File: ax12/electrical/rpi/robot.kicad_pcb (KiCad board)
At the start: 2 copper layers, 99.1 x 47 mm, 38 parts, among them J1 12V, J2 LEG1, J3 Pi USB Pwr, J4 Serial, J5 LEG2, J6 LEG3, J7 LEG4, J8 Data P, J9 Data S, U1 LM317_12, U2 AP1117-50, U3 74LS126, U4 LM317_34

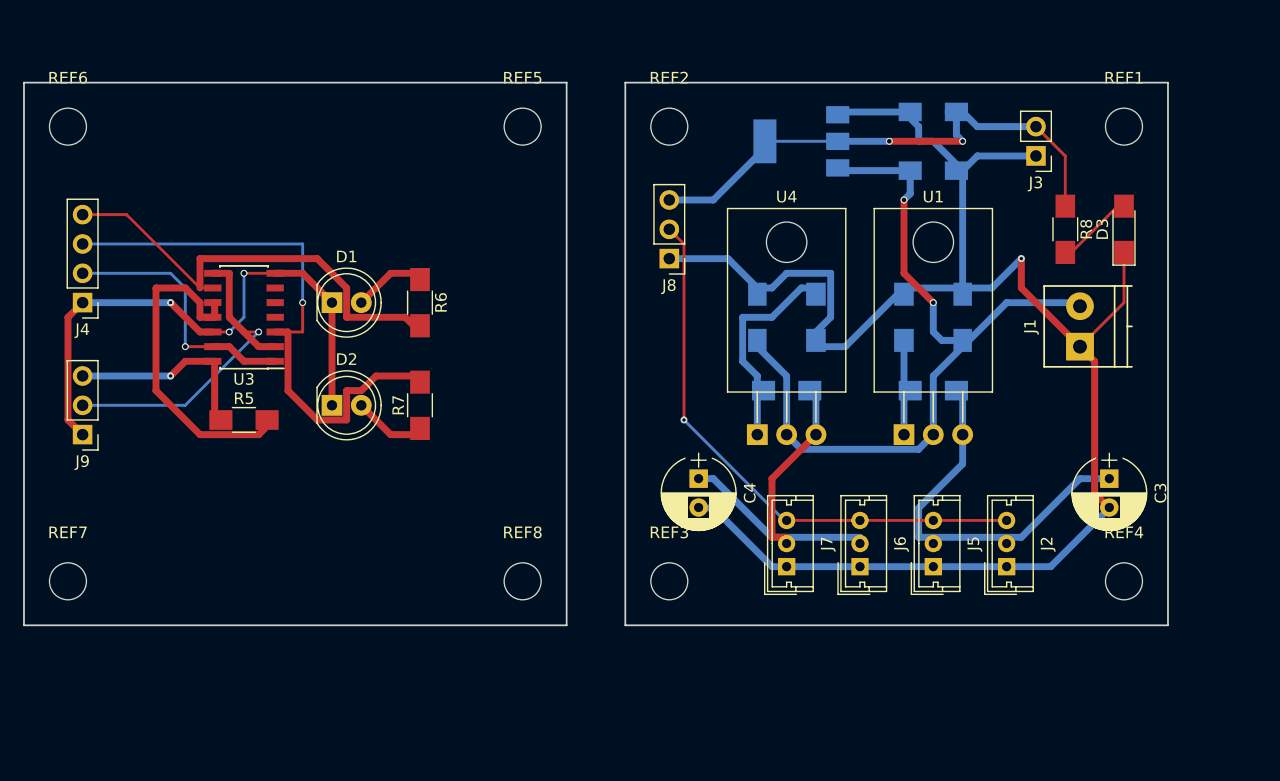
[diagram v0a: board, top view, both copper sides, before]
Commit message: update
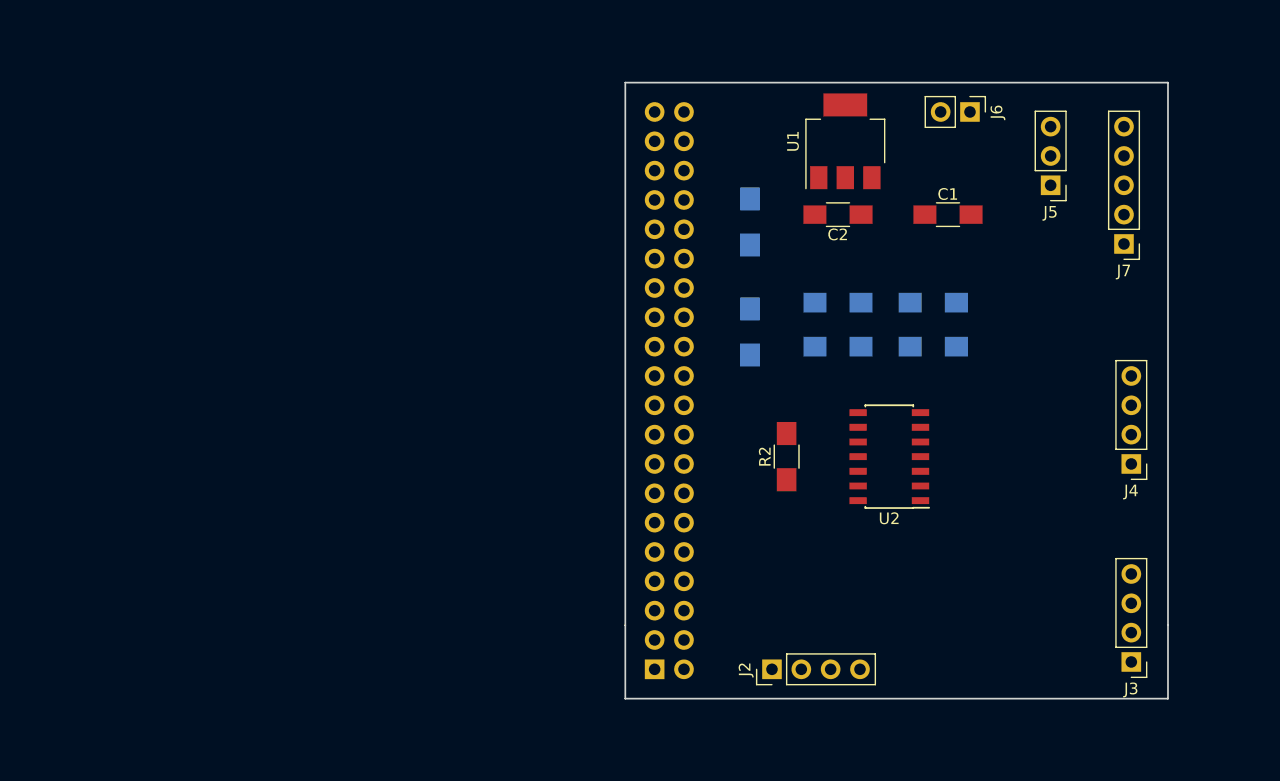
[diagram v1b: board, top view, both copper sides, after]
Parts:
- removed C3, C4: .1, Capacitors_THT:CP_Radial_D6.3mm_P2.50mm
- removed C5, C6: C, Capacitors_SMD:C_1206_HandSoldering
- removed J8: Data P, Pin_Headers:Pin_Header_Straight_1x03_Pitch2.54mm
- removed J9: Data S, Pin_Headers:Pin_Header_Straight_1x03_Pitch2.54mm
- removed R5: 10k, Resistors_SMD:R_1206_HandSoldering
- removed R6, R7, R8: 330, Resistors_SMD:R_1206_HandSoldering
- removed REF1, REF2, REF3, REF5, REF6, REF7, REF8: , Mounting_Holes:MountingHole_3.2mm_M3
- removed REF4: 3.2mm_M3, Mounting_Holes:MountingHole_3.2mm_M3
- removed U3: 74LS126, Housings_SOIC:SOIC-14_3.9x8.7mm_Pitch1.27mm
- removed U4: LM317_34, TO_SOT_Packages_THT:TO-220-3_Horizontal
- C1, C2: moved to F.Cu
- D1: value TX -> PWR; footprint LEDs:LED_D5.0mm -> LEDs:LED_1206_HandSoldering; moved to B.Cu
- D2: value RX -> TX; footprint LEDs:LED_D5.0mm -> LEDs:LED_1206_HandSoldering; moved to B.Cu
- D3: value PWR -> RX; moved to B.Cu
- J1: value 12V -> (none); footprint TerminalBlocks_Phoenix:TerminalBlock_Phoenix_PT-3.5mm_2pol -> Pin_Headers:Pin_Header_Straight_2x20_Pitch2.54mm; moved to B.Cu
- J2: value LEG1 -> IMU; footprint Connectors_Molex:Molex_MicroLatch-53253-0370_03x2.00mm_Straight -> Pin_Headers:Pin_Header_Straight_1x04_Pitch2.54mm
- J3: value Pi USB Pwr -> Lidar; footprint Pin_Headers:Pin_Header_Straight_1x02_Pitch2.54mm -> Pin_Headers:Pin_Header_Straight_1x04_Pitch2.54mm
- J5: value LEG2 -> Data S; footprint Connectors_Molex:Molex_MicroLatch-53253-0370_03x2.00mm_Straight -> Pin_Headers:Pin_Header_Straight_1x03_Pitch2.54mm
- J6: value LEG3 -> Pi USB Pwr; footprint Connectors_Molex:Molex_MicroLatch-53253-0370_03x2.00mm_Straight -> Pin_Headers:Pin_Header_Straight_1x02_Pitch2.54mm
- J7: value LEG4 -> Audio; footprint Connectors_Molex:Molex_MicroLatch-53253-0370_03x2.00mm_Straight -> Pin_Headers:Pin_Header_Straight_1x05_Pitch2.54mm
- R2: value 1.8k -> 10k; moved to F.Cu
- R4: value 1.8k -> 330
- U1: value LM317_12 -> AP1117-50; footprint TO_SOT_Packages_THT:TO-220-3_Horizontal -> TO_SOT_Packages_SMD:SOT-223-3_TabPin2
- U2: value AP1117-50 -> 74LS126; footprint TO_SOT_Packages_SMD:SOT-223-3_TabPin2 -> Housings_SOIC:SOIC-14_3.9x8.7mm_Pitch1.27mm; moved to F.Cu
- moved J4 91.9 mm to (153.0, 92.7)
- moved J1 46.2 mm to (111.8, 110.5), turned to 0 degrees
- moved D2 44.7 mm to (127.6, 78.7)
- moved J3 44.6 mm to (153.0, 109.9)
- moved J6 40.5 mm to (139.1, 62.2), turned to 270 degrees
- moved J7 40.4 mm to (152.4, 73.7), turned to 180 degrees
- moved D1 36.9 mm to (120.0, 71.8), turned to 270 degrees
- moved J5 34.5 mm to (146.1, 68.6), turned to 180 degrees
- moved U2 28.3 mm to (132.1, 92.1)
- moved D3 26.8 mm to (127.6, 82.5), turned to 0 degrees
- moved U1 25.9 mm to (128.3, 64.8), turned to 90 degrees
- moved J2 22.2 mm to (121.9, 110.5)
- moved R1 16.7 mm to (120.0, 81.3), turned to 90 degrees
- moved R2 15.8 mm to (123.2, 92.1)
- moved R3 14.8 mm to (135.9, 78.7), turned to 0 degrees
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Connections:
- C1 pad 2: GNDA -> GND
- C2 pad 2: GNDA -> GND
- D3 pad 1: GNDA -> GND
- J1 pad 1: GNDA -> Net-(J1-Pad1)
- J1 pad 2: +12V -> Net-(J1-Pad2)
- J2 pad 1: GNDA -> Net-(J1-Pad17)
- J2 pad 2: /PWR12 -> Net-(J1-Pad3)
- J2 pad 3: /DATA -> Net-(J1-Pad5)
- J3 pad 1: GNDA -> +5V
- J3 pad 2: +5V -> Net-(J1-Pad8)
- J5 pad 1: GNDA -> GND
- J5 pad 2: /PWR12 -> Net-(J5-Pad2)
- J5 pad 3: /DATA -> +12V
- J6 pad 1: GNDA -> GND
- J6 pad 2: /PWR34 -> +5V
- J7 pad 1: GNDA -> Net-(J7-Pad1)
- J7 pad 2: /PWR34 -> Net-(J7-Pad2)
- J7 pad 3: /DATA -> Net-(J7-Pad3)
- R1 pad 1: /PWR12 -> +5V
- R1 pad 2: Net-(R1-Pad2) -> Net-(D1-Pad2)
- R2 pad 1: Net-(R1-Pad2) -> +5V
- R2 pad 2: GNDA -> Net-(R2-Pad2)
- R3 pad 1: /PWR34 -> Net-(D2-Pad2)
- R3 pad 2: Net-(R3-Pad2) -> /TXI
- R4 pad 1: Net-(R3-Pad2) -> Net-(D3-Pad2)
- R4 pad 2: GNDA -> /RXO
- U1 pad 1: Net-(R1-Pad2) -> GND
- U1 pad 2: +12V -> +5V
- U1 pad 3: /PWR12 -> +12V
- U2 pad 1: GNDA -> /DTR
- U2 pad 2: +5V -> Net-(J5-Pad2)
- U2 pad 3: +12V -> /RXO
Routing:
- net GNDA: track 157.3 -> 0.00 mm, vias 1 -> 0
- net +12V: track 71.5 -> 0.00 mm, vias 2 -> 0
- net /RXO: track 51.3 -> 0.00 mm, vias 1 -> 0
- net +5V: track 49.5 -> 0.00 mm, vias 2 -> 0
- net GND: track 49.4 -> 0.00 mm, vias 3 -> 0
- net /DATA: track 48.8 -> 0.00 mm, vias 1 -> 0
- net /TXI: track 40.1 -> 0.00 mm
- net /PWR12: track 35.6 -> 0.00 mm
- net /PWR34: track 34.3 -> 0.00 mm
- net Net-(R5-Pad2): track 30.0 -> 0.00 mm
- net Net-(J9-Pad2): track 29.4 -> 0.00 mm, vias 1 -> 0
- net /DTR: track 22.8 -> 0.00 mm, vias 1 -> 0
- net Net-(R3-Pad2): track 19.7 -> 0.00 mm
- net +5VA: track 17.6 -> 0.00 mm, vias 1 -> 0
- net Net-(R1-Pad2): track 9.24 -> 0.00 mm
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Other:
- board size 99.1 x 47 mm -> 47 x 53.3 mm

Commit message: electrical update
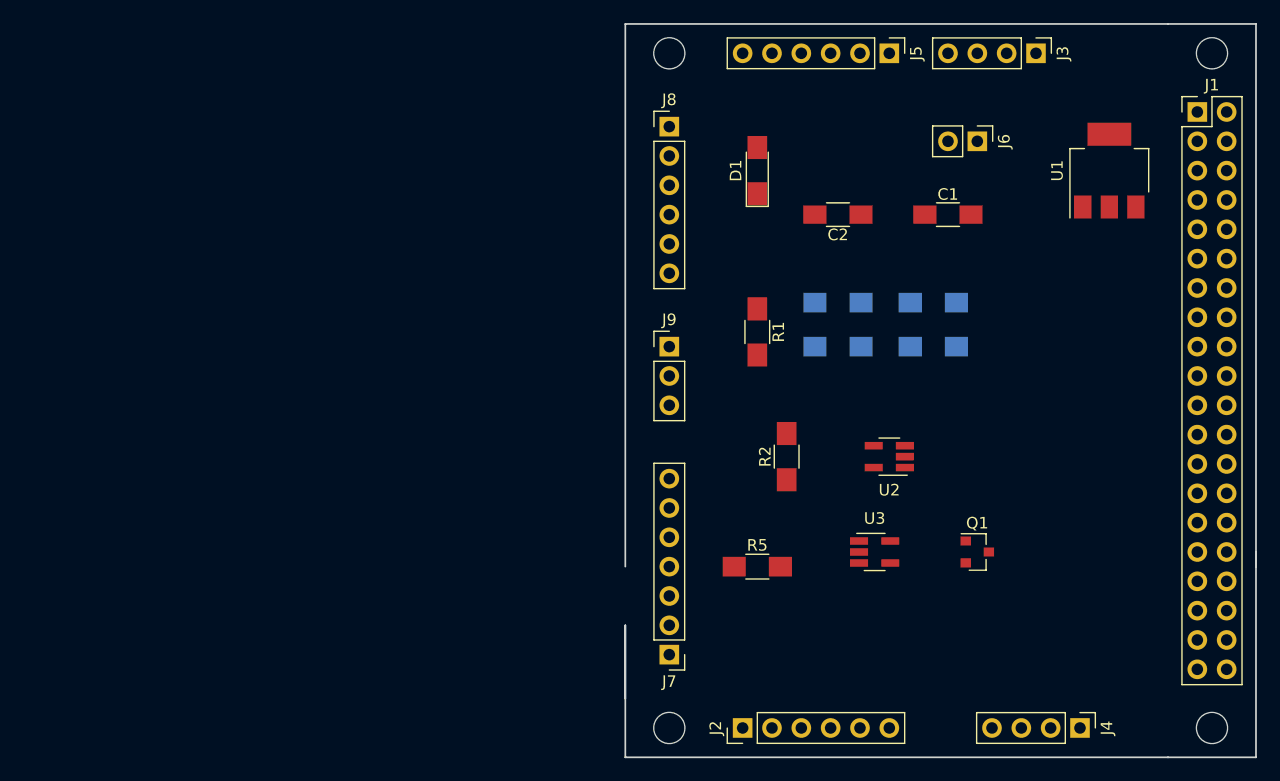
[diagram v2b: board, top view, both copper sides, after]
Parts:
- added J8: SERIAL, Pin_Headers:Pin_Header_Straight_1x06_Pitch2.54mm, F.Cu at (113.0, 63.5)
- added J9: PWR BOARD, Pin_Headers:Pin_Header_Straight_1x03_Pitch2.54mm, F.Cu at (113.0, 82.5)
- added Q1: BSS138, TO_SOT_Packages_SMD:SOT-23, F.Cu at (139.7, 100.3)
- added R5: 330, Resistors_SMD:R_1206_HandSoldering, F.Cu at (120.7, 101.6)
- added REF**: MountingHole_2.7mm, Mounting_Holes:MountingHole_2.7mm, F.Cu at (113.0, 115.6)
- added REF**: MountingHole_2.7mm, Mounting_Holes:MountingHole_2.7mm, F.Cu at (113.0, 57.1)
- added REF**: MountingHole_2.7mm, Mounting_Holes:MountingHole_2.7mm, F.Cu at (160.0, 115.6)
- added REF**: MountingHole_2.7mm, Mounting_Holes:MountingHole_2.7mm, F.Cu at (160.0, 57.1)
- added U3: 74LVC1G126, TO_SOT_Packages_SMD:SOT-23-5_HandSoldering, F.Cu at (130.8, 100.3)
- D1, R1: moved to F.Cu
- J1: value (none) -> Raspberry_Pi_2_3; moved to F.Cu
- J2: footprint Pin_Headers:Pin_Header_Straight_1x04_Pitch2.54mm -> Pin_Headers:Pin_Header_Straight_1x06_Pitch2.54mm
- J4: value Serial -> I2C
- J5: value Data S -> SPI; footprint Pin_Headers:Pin_Header_Straight_1x03_Pitch2.54mm -> Pin_Headers:Pin_Header_Straight_1x06_Pitch2.54mm
- J7: footprint Pin_Headers:Pin_Header_Straight_1x05_Pitch2.54mm -> Pin_Headers:Pin_Header_Straight_1x07_Pitch2.54mm
- R2: value 10k -> 330
- U2: value 74LS126 -> 74LVC1G125; footprint Housings_SOIC:SOIC-14_3.9x8.7mm_Pitch1.27mm -> TO_SOT_Packages_SMD:SOT-23-5_HandSoldering
- moved J1 67.4 mm to (158.8, 62.2)
- moved J3 53.3 mm to (144.8, 57.1), turned to 270 degrees
- moved J7 53.1 mm to (113.0, 109.2)
- moved J4 23.3 mm to (148.6, 115.6), turned to 270 degrees
- moved U1 23.0 mm to (151.1, 67.3)
- moved J5 18.1 mm to (132.1, 57.1), turned to 270 degrees
- moved J2 5.68 mm to (119.4, 115.6)
- moved D1 4.49 mm to (120.7, 67.3), turned to 90 degrees
- moved J6 2.62 mm to (139.7, 64.8)
- moved R1 0.64 mm to (120.7, 81.3), turned to 270 degrees
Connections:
- D2 pad 1: GND -> Net-(D2-Pad1)
- D2 pad 2: Net-(D2-Pad2) -> +3V3
- D3 pad 1: GND -> Net-(D3-Pad1)
- D3 pad 2: Net-(D3-Pad2) -> RXI
- J1 pad 1: Net-(J1-Pad1) -> +3V3
- J1 pad 12: Net-(J1-Pad12) -> BCLK
- J1 pad 19: Net-(J1-Pad19) -> MOSI
- J1 pad 21: Net-(J1-Pad21) -> MISO
- J1 pad 23: Net-(J1-Pad23) -> SPI-CLK
- J1 pad 24: Net-(J1-Pad24) -> CS
- J1 pad 29: Net-(J1-Pad29) -> IMU-RST
- J1 pad 35: Net-(J1-Pad35) -> LRC
- J1 pad 40: Net-(J1-Pad40) -> DIN
- J2 pad 1: Net-(J1-Pad17) -> +3V3
- J2 pad 2: Net-(J1-Pad3) -> Net-(J2-Pad2)
- J2 pad 3: Net-(J1-Pad5) -> GND
- J2 pad 4: GND -> Net-(J1-Pad5)
- J4 pad 1: GND -> +3V3
- J4 pad 2: /DTR -> GND
- J4 pad 3: /RXO -> Net-(J1-Pad3)
- J4 pad 4: /TXI -> Net-(J1-Pad5)
- J5 pad 1: GND -> +3V3
- J5 pad 2: Net-(J5-Pad2) -> GND
- J5 pad 3: +12V -> CS
- J7 pad 1: Net-(J7-Pad1) -> LRC
- J7 pad 2: Net-(J7-Pad2) -> BCLK
- J7 pad 3: Net-(J7-Pad3) -> DIN
- R2 pad 2: Net-(R2-Pad2) -> DATA
- R3 pad 1: Net-(D2-Pad2) -> +3V3
- R3 pad 2: /TXI -> DTR
- R4 pad 1: Net-(D3-Pad2) -> Net-(D2-Pad1)
- R4 pad 2: /RXO -> TXO
- U2 pad 1: /DTR -> DTR
- U2 pad 2: Net-(J5-Pad2) -> TXO
- U2 pad 3: /RXO -> GND
- U2 pad 4: /DTR -> DTR
- U2 pad 5: GND -> +3V3
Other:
- board size 47 x 53.3 mm -> 54.6 x 63.5 mm
